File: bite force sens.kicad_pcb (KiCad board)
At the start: 2 copper layers, 31.5 x 75 mm, 20 parts, among them J1 Flexiforce, J2 oled display, J4 switch, J6 Conn_01x02, J7 Conn_01x02, U1 XIAO ESP32 S3, U2 MCP6004

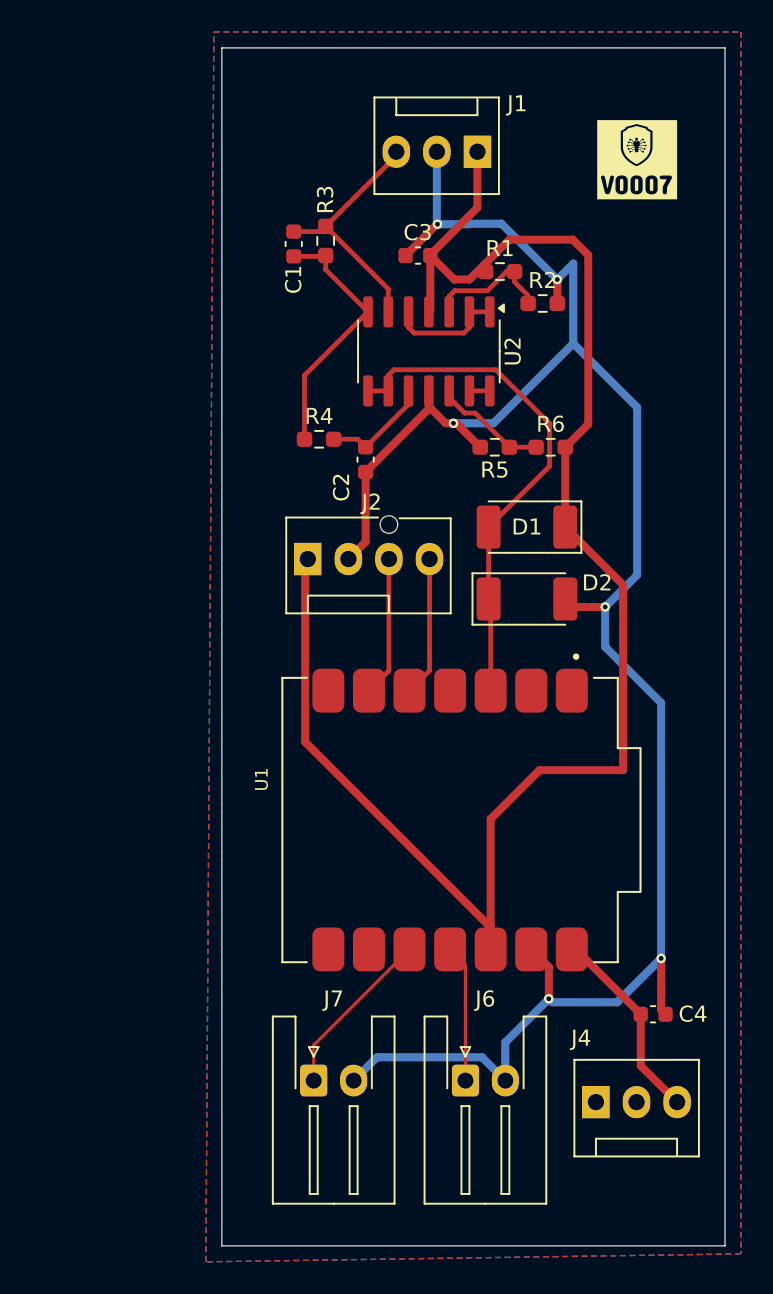
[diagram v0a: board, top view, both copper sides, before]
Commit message: made entire change in design and now the fresh pcb will be done and comitted at next commit
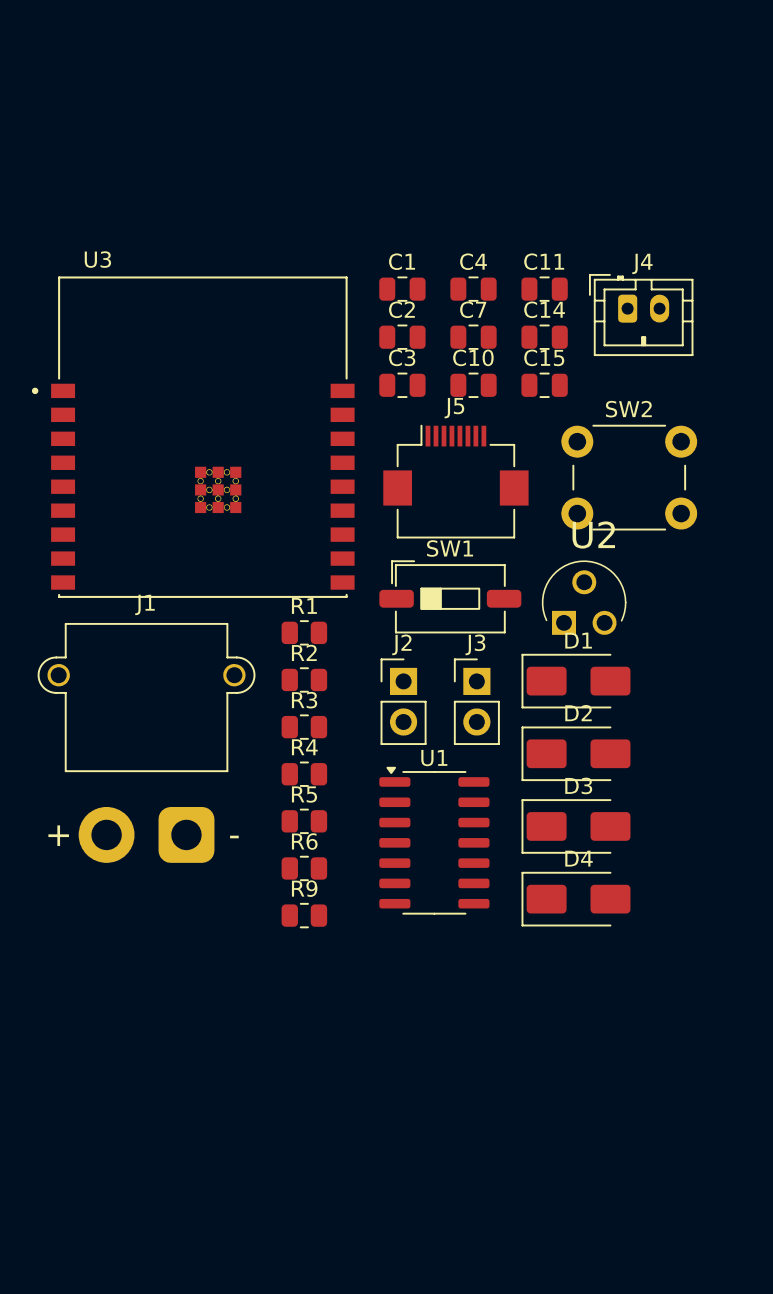
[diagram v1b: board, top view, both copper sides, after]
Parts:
- removed J6, J7: Conn_01x02, Connector_JST:JST_XH_S2B-XH-A-1_1x02_P2.50mm_Horizontal
- removed a: LOGO, LOGO
- added C10: 10u, Capacitor_SMD:C_0805_2012Metric, F.Cu at (155.3, 81.6)
- added C11: 47p, Capacitor_SMD:C_0805_2012Metric, F.Cu at (159.7, 75.6)
- added C14: C, Capacitor_SMD:C_0805_2012Metric, F.Cu at (159.7, 78.6)
- added C15: 0.1u, Capacitor_SMD:C_0805_2012Metric, F.Cu at (159.7, 81.6)
- added C7: 47p, Capacitor_SMD:C_0805_2012Metric, F.Cu at (155.3, 78.6)
- added D3: D_Zener, Diode_SMD:D_SMA, F.Cu at (161.8, 109.2)
- added D4: D_Schottky, Diode_SMD:D_SMA, F.Cu at (161.8, 113.8)
- added J3: tp4056 pin, Connector_PinHeader_2.54mm:PinHeader_1x02_P2.54mm_Vertical, F.Cu at (155.5, 100.2)
- added J5: display, connec:Hirose_FH12-8S-0.5SH_1x08-1MP_P0.50mm_Horizontal, F.Cu at (154.2, 86.7)
- added R9: 100k, Resistor_SMD:R_0805_2012Metric, F.Cu at (144.7, 114.8)
- added SW1: on/off, Button_Switch_SMD:SW_DIP_SPSTx01_Slide_6.7x4.1mm_W6.73mm_P2.54mm_LowProfile_JPin, F.Cu at (153.8, 95.0)
- added SW2: reset, Button_Switch_THT:SW_PUSH_6mm, F.Cu at (161.8, 85.2)
- added U3: ESP32-C3-WROOM-02-N4, esp32 footrpint:MODULE_ESP32-C3-WROOM-02-H4, F.Cu at (138.3, 84.9)
- C1, C2: value 47p -> 10u; footprint Capacitor_SMD:C_0603_1608Metric -> Capacitor_SMD:C_0805_2012Metric
- C3, C4: footprint Capacitor_SMD:C_0603_1608Metric -> Capacitor_SMD:C_0805_2012Metric
- D1, D2: value 1N5711UR -> D_Schottky; footprint Diode_SMD:D_MELF -> Diode_SMD:D_SMA
- J1: value Flexiforce -> lipo bat; footprint Connector:FanPinHeader_1x03_P2.54mm_Vertical -> Connector_AMASS:AMASS_XT30PW-M_1x02_P2.50mm_Horizontal
- J2: value oled display -> tp4056 pin; footprint Connector:FanPinHeader_1x04_P2.54mm_Vertical -> Connector_PinHeader_2.54mm:PinHeader_1x02_P2.54mm_Vertical
- J4: value switch -> fsr; footprint Connector:FanPinHeader_1x03_P2.54mm_Vertical -> Connector_JST:JST_PH_B2B-PH-K_1x02_P2.00mm_Vertical
- R1: value 80k -> 20k; footprint Resistor_SMD:R_0603_1608Metric_Pad0.98x0.95mm_HandSolder -> Resistor_SMD:R_0805_2012Metric
- R2: value 20k -> 80k; footprint Resistor_SMD:R_0603_1608Metric_Pad0.98x0.95mm_HandSolder -> Resistor_SMD:R_0805_2012Metric
- R3: value 100k -> 10k; footprint Resistor_SMD:R_0603_1608Metric_Pad0.98x0.95mm_HandSolder -> Resistor_SMD:R_0805_2012Metric
- R4, R6: footprint Resistor_SMD:R_0603_1608Metric_Pad0.98x0.95mm_HandSolder -> Resistor_SMD:R_0805_2012Metric
- R5: value 10k -> 33; footprint Resistor_SMD:R_0603_1608Metric_Pad0.98x0.95mm_HandSolder -> Resistor_SMD:R_0805_2012Metric
- U1: value XIAO ESP32 S3 -> MCP6004; footprint XIAO_Footprints:MODULE_102010428 -> Package_SO:SOIC-14_3.9x8.7mm_P1.27mm
- U2: value MCP6004 -> MCP1700-3302E_TO; footprint Package_SO:SOIC-14_3.9x8.7mm_P1.27mm -> mcp1700:TO127P254X495-3
- moved J4 49.7 mm to (164.9, 76.8)
- moved C4 46.8 mm to (155.3, 75.6), turned to 0 degrees
- moved J1 46.5 mm to (137.3, 109.8), turned to 0 degrees
- moved R6 30.6 mm to (144.7, 111.9)
- moved R3 30.5 mm to (144.7, 103.0), turned to 0 degrees
- moved R2 27.9 mm to (144.7, 100.1)
- moved R5 26.3 mm to (144.7, 108.9), turned to 0 degrees
- moved R1 25.7 mm to (144.7, 97.1)
- moved R4 21.0 mm to (144.7, 106.0)
- moved U2 18.2 mm to (163.5, 94.0), turned to 0 degrees
- moved D2 10.2 mm to (161.8, 104.7)
- moved D1 10.2 mm to (161.8, 100.1), turned to 0 degrees
- moved J2 9.73 mm to (150.9, 100.2)
- moved C3 8.18 mm to (150.8, 81.6)
- moved C2 8.00 mm to (150.8, 78.6), turned to 0 degrees
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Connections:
- C1 pad 1: Net-(J1-Pin_3) -> GND
- C1 pad 2: Net-(C1-Pad2) -> /v
- C2 pad 1: GND -> /3.3
- C2 pad 2: Net-(U2C-+) -> GND
- C3 pad 2: /3v3 -> /v
- C4 pad 2: Net-(J4-Pin_3) -> /3v3
- D1 pad 1: /3v3 -> /V3
- D1 pad 2: /Sensor Output -> GND
- D2 pad 1: /Sensor Output -> /+
- J1 pad 1: /3v3 -> /-
- J1 pad 2: GND -> /+
- J2 pad 1: /3v3 -> /v
- J2 pad 2: GND -> /+
- J4 pad 1: unconnected-(J4-Pin_1-Pad1) -> Net-(J4-Pin_1)
- J4 pad 2: +5V -> GND
- R1 pad 1: /3v3 -> /v0
- R1 pad 2: Net-(U2A-+) -> GND
- R2 pad 1: Net-(U2A-+) -> /3v3
- R2 pad 2: GND -> /v0
- R3 pad 1: Net-(J1-Pin_3) -> /v2
- R3 pad 2: Net-(C1-Pad2) -> Net-(U1C-+)
- R4 pad 1: Net-(C1-Pad2) -> Net-(U1D-+)
- R4 pad 2: Net-(U2C-+) -> /3v3
- R5 pad 1: Net-(U2D-+) -> Net-(J5-Pin_1)
- R5 pad 2: GND -> /3v3
- R6 pad 1: Net-(U2D-+) -> GND
- R6 pad 2: /3v3 -> Net-(U1D-+)
- U1 pad 1: unconnected-(U1-P26/A0/D0-Pad1) -> /v1
- U1 pad 10: Net-(J7-Pin_1) -> Net-(U1C-+)
- U1 pad 11: Net-(J6-Pin_1) -> GND
- U1 pad 12: /3v3 -> Net-(U1D-+)
- U1 pad 13: GND -> Net-(U1D--)
- U1 pad 14: Net-(J4-Pin_3) -> Net-(U1D--)
- U1 pad 2: unconnected-(U1-P27/A1/D1-Pad2) -> /v1
- U1 pad 3: /Sensor Output -> /v0
- U1 pad 4: unconnected-(U1-P29/A3/D3-Pad4) -> /3v3
- U1 pad 5: Net-(J2-Pin_4) -> /v1
- U1 pad 6: Net-(J2-Pin_3) -> Net-(J4-Pin_1)
- U1 pad 7: unconnected-(U1-P0//TX/D6-Pad7) -> /v2
- U1 pad 8: unconnected-(U1-D7/CSB/P1/RX-Pad8) -> /V3
- U1 pad 9: unconnected-(U1-D8/SCK/P2-Pad9) -> /V3
- U2 pad 1: Net-(U2A--) -> GND
- U2 pad 2: Net-(U2A--) -> /v
- U2 pad 3: Net-(U2A-+) -> /3.3
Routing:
- net GND: track 129.2 -> 0.00 mm, vias 6 -> 0
- net /3v3: track 104.6 -> 0.00 mm
- net /Sensor Output: track 32.2 -> 0.00 mm
- net Net-(C1-Pad2): track 16.3 -> 0.00 mm
- net Net-(J1-Pin_3): track 15.2 -> 0.00 mm
- net Net-(J4-Pin_3): track 12.4 -> 0.00 mm
- net Net-(J7-Pin_1): track 10.7 -> 0.00 mm
- net Net-(J2-Pin_4): track 8.76 -> 0.00 mm
- net Net-(J2-Pin_3): track 8.76 -> 0.00 mm
- net Net-(J6-Pin_1): track 8.61 -> 0.00 mm
- net Net-(U2A-+): track 7.56 -> 0.00 mm
- net Net-(U2A--): track 7.32 -> 0.00 mm
- net Net-(U2D-+): track 7.15 -> 0.00 mm
- net Net-(U2C-+): track 6.85 -> 0.00 mm
- net Net-(U2D--): track 1.27 -> 0.00 mm
- removed copper zone on B.Cu, net GND
- removed copper zone on F.Cu, net GND
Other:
- board outline removed
